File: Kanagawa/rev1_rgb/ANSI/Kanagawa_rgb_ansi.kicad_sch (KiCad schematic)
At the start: 187 parts, among them J1 Oled128x64, J3 OledJump2, J4 OledJump1, J5 RGB_Out, J6 RGB_Selector_Pin, J7 RGB_Selector_Matrix, SW99 Rotary_Encoder_Switch, U0 Elite-C

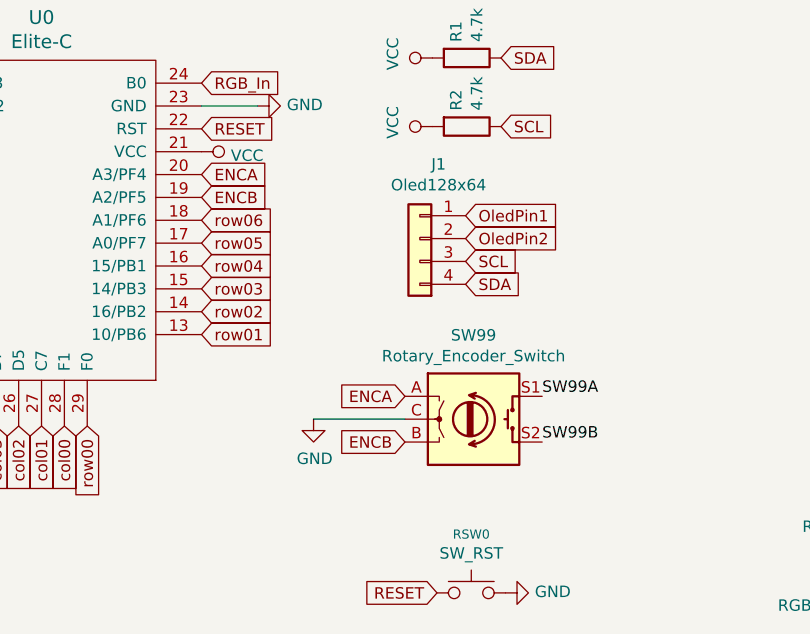
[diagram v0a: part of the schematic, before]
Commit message: restart RGB
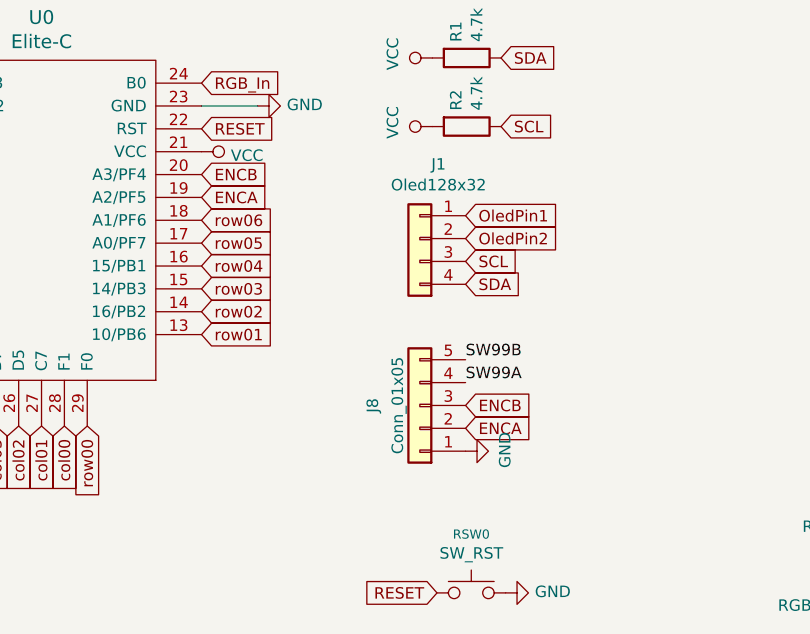
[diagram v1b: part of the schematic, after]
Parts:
- removed SW99: Rotary_Encoder_Switch, keyboard:RotaryEncoder_Alps_EC11E-Switch_Vertical_H20mm, symbol keyboard:Rotary_Encoder_Switch
- added J8: Conn_01x05, keyboard:PinHeader_1x05_P2.54mm_Vertical, symbol keyboard:Conn_01x05
- J1: value Oled128x64 -> Oled128x32; footprint keyboard:OLED_128x64_I2C_cutout -> keyboard:OLED_128x32_I2C
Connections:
- net ENCA: now also U0.19 (A2/PF5), J8.2 (Pin_2); no longer U0.20 (A3/PF4)
- net ENCB: now also U0.20 (A3/PF4), J8.3 (Pin_3); no longer U0.19 (A2/PF5)
- net GND: now also J8.1 (Pin_1)
- net SW99B: now also J8.5 (Pin_5)
- net col11: now also J8.4 (Pin_4)
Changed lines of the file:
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@@
     (stroke (width 0) (type default) (color 0 0 0 0))
   )
-  (wire (pts (xy 73.152 58.928) (xy 83.312 58.928))
-    (stroke (width 0) (type default) (color 0 0 0 0))
-  )
   (wire (pts (xy 57.404 203.708) (xy 57.404 208.534))
     (stroke (width 0) (type default) (color 0 0 0 0))
@@
     (effects (font (size 1.27 1.27)) (justify left bottom))
   )
-  (label "SW99B" (at 98.552 61.468 0)
+  (label "SW99B" (at 90.043 52.324 0)
     (effects (font (size 1.27 1.27)) (justify left bottom))
   )
@@
     (effects (font (size 1.27 1.27)) (justify left bottom))
   )
-  (label "SW99A" (at 98.552 56.388 0)
+  (label "SW99A" (at 90.043 54.864 0)
     (effects (font (size 1.27 1.27)) (justify left bottom))
   )
@@
     )
   )
-  (global_label "ENCA" (shape input) (at 60.706 31.75 0) (fields_autoplaced)
+  (global_label "ENCA" (shape input) (at 60.706 34.29 0) (fields_autoplaced)
     (effects (font (size 1.27 1.27)) (justify left))
-    (property "Intersheet References" "${INTERSHEET_REFS}" (id 0) (at 0 10.16 0)
+    (property "Intersheet References" "${INTERSHEET_REFS}" (id 0) (at 0 12.7 0)
       (effects (font (size 1.27 1.27)) hide)
     )
@@
     )
   )
-  (global_label "ENCB" (shape input) (at 60.706 34.29 0) (fields_autoplaced)
+  (global_label "ENCB" (shape input) (at 60.706 31.75 0) (fields_autoplaced)
     (effects (font (size 1.27 1.27)) (justify left))
-    (property "Intersheet References" "${INTERSHEET_REFS}" (id 0) (at 0 2.54 0)
+    (property "Intersheet References" "${INTERSHEET_REFS}" (id 0) (at 0 0 0)
       (effects (font (size 1.27 1.27)) hide)
     )
@@
     )
   )
-  (global_label "ENCB" (shape input) (at 83.312 61.468 180) (fields_autoplaced)
-    (effects (font (size 1.27 1.27)) (justify right))
-    (property "Intersheet References" "${INTERSHEET_REFS}" (id 0) (at 0 0 0)
+  (global_label "ENCB" (shape input) (at 90.043 57.404 0) (fields_autoplaced)
+    (effects (font (size 1.27 1.27)) (justify left))
+    (property "Intersheet References" "${INTERSHEET_REFS}" (id 0) (at 173.355 118.872 0)
       (effects (font (size 1.27 1.27)) hide)
     )
@@
     )
   )
-  (global_label "ENCA" (shape input) (at 83.312 56.388 180) (fields_autoplaced)
-    (effects (font (size 1.27 1.27)) (justify right))
-    (property "Intersheet References" "${INTERSHEET_REFS}" (id 0) (at 0 0 0)
+  (global_label "ENCA" (shape input) (at 90.043 59.944 0) (fields_autoplaced)
+    (effects (font (size 1.27 1.27)) (justify left))
+    (property "Intersheet References" "${INTERSHEET_REFS}" (id 0) (at 173.355 116.332 0)
       (effects (font (size 1.27 1.27)) hide)
     )
@@
     )
   )
-  (symbol (lib_id "keyboard:Rotary_Encoder_Switch") (at 90.932 58.928 0) (unit 1)
-    (in_bom yes) (on_board yes)
-    (property "Reference" "SW99" (id 0) (at 90.932 49.6062 0))
-    (property "Value" "Rotary_Encoder_Switch" (id 1) (at 90.932 51.9176 0))
-    (property "Footprint" "keyboard:RotaryEncoder_Alps_EC11E-Switch_Vertical_H20mm" (id 2) (at 99.822 67.564 0)
-      (effects (font (size 1.27 1.27)) hide)
-    )
-    (property "Datasheet" "" (id 3) (at 90.932 52.324 0)
-      (effects (font (size 1.27 1.27)) hide)
-    )
-    (pin "A")
-    (pin "B")
-    (pin "C")
-    (pin "S1")
-    (pin "S2")
-  )
   (symbol (lib_name "KEY_SW_RGB_13") (lib_id "keyboard:KEY_SW_RGB") (at 43.434 196.088 0) (unit 1)
     (in_bom yes) (on_board yes)
@@
     (pin "6")
   )
-  (symbol (lib_id "keyboard:GND") (at 73.152 58.928 0) (unit 1)
+  (symbol (lib_id "keyboard:GND") (at 90.043 62.484 90) (unit 1)
     (in_bom yes) (on_board yes)
-    (property "Reference" "#PWR0111" (id 0) (at 73.152 65.278 0)
+    (property "Reference" "#PWR0111" (id 0) (at 96.393 62.484 0)
       (effects (font (size 1.27 1.27)) hide)
     )
-    (property "Value" "GND" (id 1) (at 73.279 63.3222 0))
-    (property "Footprint" "" (id 2) (at 73.152 58.928 0)
+    (property "Value" "GND" (id 1) (at 94.4372 62.357 0))
+    (property "Footprint" "" (id 2) (at 90.043 62.484 0)
       (effects (font (size 1.27 1.27)) hide)
     )
-    (property "Datasheet" "" (id 3) (at 73.152 58.928 0)
+    (property "Datasheet" "" (id 3) (at 90.043 62.484 0)
       (effects (font (size 1.27 1.27)) hide)
     )
@@
     (in_bom yes) (on_board yes)
     (property "Reference" "J1" (id 0) (at 87.0458 30.607 0))
-    (property "Value" "Oled128x64" (id 1) (at 87.0458 32.9184 0))
-    (property "Footprint" "keyboard:OLED_128x64_I2C_cutout" (id 2) (at 81.153 31.242 0)
+    (property "Value" "Oled128x32" (id 1) (at 87.0458 32.9184 0))
+    (property "Footprint" "keyboard:OLED_128x32_I2C" (id 2) (at 81.153 31.242 0)
       (effects (font (size 1.27 1.27)) hide)
     )
@@
     (pin "3")
   )
+  (symbol (lib_id "keyboard:Conn_01x05") (at 84.963 57.404 180) (unit 1)
+    (in_bom yes) (on_board yes) (fields_autoplaced)
+    (property "Reference" "J8" (id 0) (at 79.7265 57.404 90))
+    (property "Value" "Conn_01x05" (id 1) (at 82.5016 57.404 90))
+    (property "Footprint" "keyboard:PinHeader_1x05_P2.54mm_Vertical" (id 2) (at 84.963 57.404 0)
+      (effects (font (size 1.27 1.27)) hide)
+    )
+    (property "Datasheet" "~" (id 3) (at 84.963 57.404 0)
+      (effects (font (size 1.27 1.27)) hide)
+    )
+    (pin "1")
+    (pin "2")
+    (pin "3")
+    (pin "4")
+    (pin "5")
+  )
   (symbol (lib_id "keyboard:VCC") (at 139.954 35.687 90) (unit 1)
     (in_bom yes) (on_board yes)
@@
     )
     (path "/00000000-0000-0000-0000-0000751ebd82"
-      (reference "J1") (unit 1) (value "Oled128x64") (footprint "keyboard:OLED_128x64_I2C_cutout")
+      (reference "J1") (unit 1) (value "Oled128x32") (footprint "keyboard:OLED_128x32_I2C")
     )
     (path "/6c743fff-5b14-4739-9941-bdd029d274b2"
@@
       (reference "J7") (unit 1) (value "RGB_Selector_Matrix") (footprint "keyboard:Jumper_2pins")
     )
+    (path "/7d178fab-a20b-43c5-b3d5-8fb17e7d08a1"
+      (reference "J8") (unit 1) (value "Conn_01x05") (footprint "keyboard:PinHeader_1x05_P2.54mm_Vertical")
+    )
     (path "/00000000-0000-0000-0000-000061301752"
       (reference "KA0") (unit 1) (value "KEY_SW") (footprint "keyboard:SW_Cherry_MX_1.00u_SK6812MINI")
@@
       (reference "RSW0") (unit 1) (value "SW_RST") (footprint "keyboard:SW_RST")
     )
-    (path "/00000000-0000-0000-0000-0000612f6729"
-      (reference "SW99") (unit 1) (value "Rotary_Encoder_Switch") (footprint "keyboard:RotaryEncoder_Alps_EC11E-Switch_Vertical_H20mm")
-    )
     (path "/00000000-0000-0000-0000-0000614e8e91"

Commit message: edit kanagawa rgb
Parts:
- removed U0: Elite-C, keyboard:Elite-C-29pin-holes, symbol keyboard:Elite-C
- added U1: Pico, keyboard:RPi_Pico_TH, symbol keyboard:Pico
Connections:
- net ENCA: now also U1.31 (GPIO26_ADC0)
- net ENCB: now also U1.32 (GPIO27_ADC1)
- net GND: now also U1.13 (GND), U1.18 (GND), U1.23 (GND), U1.28 (GND), U1.3 (GND), U1.33 (AGND), U1.38 (GND), U1.8 (GND)
- net RESET: now also U1.30 (RUN)
- net SCL: now also U1.2 (GPIO1)
- net SDA: now also U1.1 (GPIO0)
- net VCC: now also U1.36 (3V3)
- net col00: now also U1.4 (GPIO2); no longer KD13.1
- net col01: now also U1.5 (GPIO3); no longer KE13.1
- net col02: now also U1.6 (GPIO4); no longer KF13.1
- net col03: now also U1.7 (GPIO5); no longer KF12.1
- net col04: now also U1.9 (GPIO6); no longer KE12.1
- net col05: now also U1.10 (GPIO7); no longer KD12.1
- net col06: now also U1.11 (GPIO8); no longer KC13.1
- net col07: now also U1.12 (GPIO9); no longer KC12.1
- net col08: now also U1.14 (GPIO10); no longer KB12.1
- net col09: now also U1.15 (GPIO11); no longer KB13.1
- net col10: now also U1.16 (GPIO12); no longer KA12.1
- net col11: now also U1.17 (GPIO13); no longer J8.4 (Pin_4)
- net row00: now also DA12.1 (K), DA13.1 (K), U1.22 (GPIO17)
- net row01: now also DB12.1 (K), DB13.1 (K), U1.24 (GPIO18)
- net row02: now also DC12.1 (K), DC13.1 (K), U1.25 (GPIO19)
- net row03: now also DD12.1 (K), DD13.1 (K), U1.26 (GPIO20)
- net row04: now also DE12.1 (K), DE13.1 (K), U1.27 (GPIO21)
- net row05: now also DF12.1 (K), DF13.1 (K), U1.29 (GPIO22)
- net RGB_In renamed RGB
- net RGB: now also U1.34 (GPIO28_ADC2)
- removed net row06: DA12.1 (K), DA13.1 (K), DB12.1 (K), DB13.1 (K), DC12.1 (K), DC13.1 (K), DD12.1 (K), DD13.1 (K), DE12.1 (K), DE13.1 (K), DF12.1 (K), DF13.1 (K)
- new net col12: KA12.1, KB12.1, KC12.1, KD12.1, KE12.1, KF12.1, U1.19 (GPIO14)
- new net col13: J8.4 (Pin_4), KB13.1, KC13.1, KD13.1, KE13.1, KF13.1, U1.21 (GPIO16)
- no-connect marks 0 -> 8
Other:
- moved on the sheet: DA0, DA1, DA10, DA11, DA12, DA13, DA2, DA3, DA4, DA5, DA6, DA7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
